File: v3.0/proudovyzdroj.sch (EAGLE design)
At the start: 27 parts, among them IC1 LM358N, Q1 IRF512

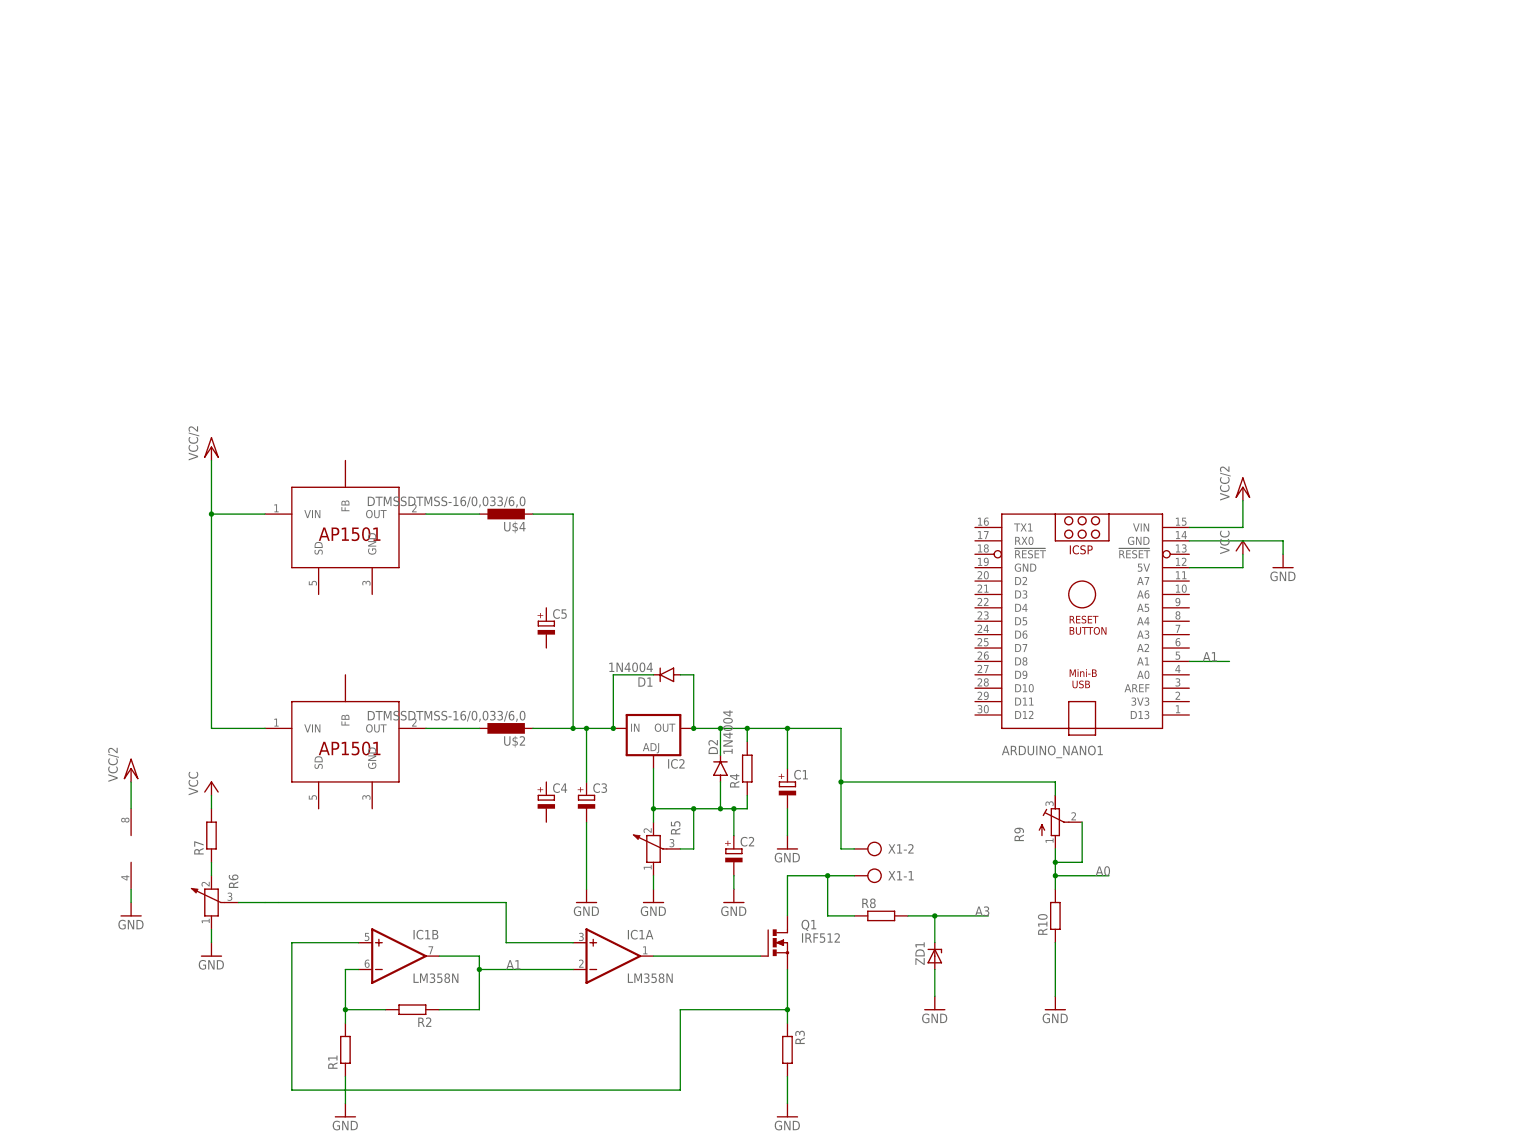
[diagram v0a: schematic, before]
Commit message: základní schéma
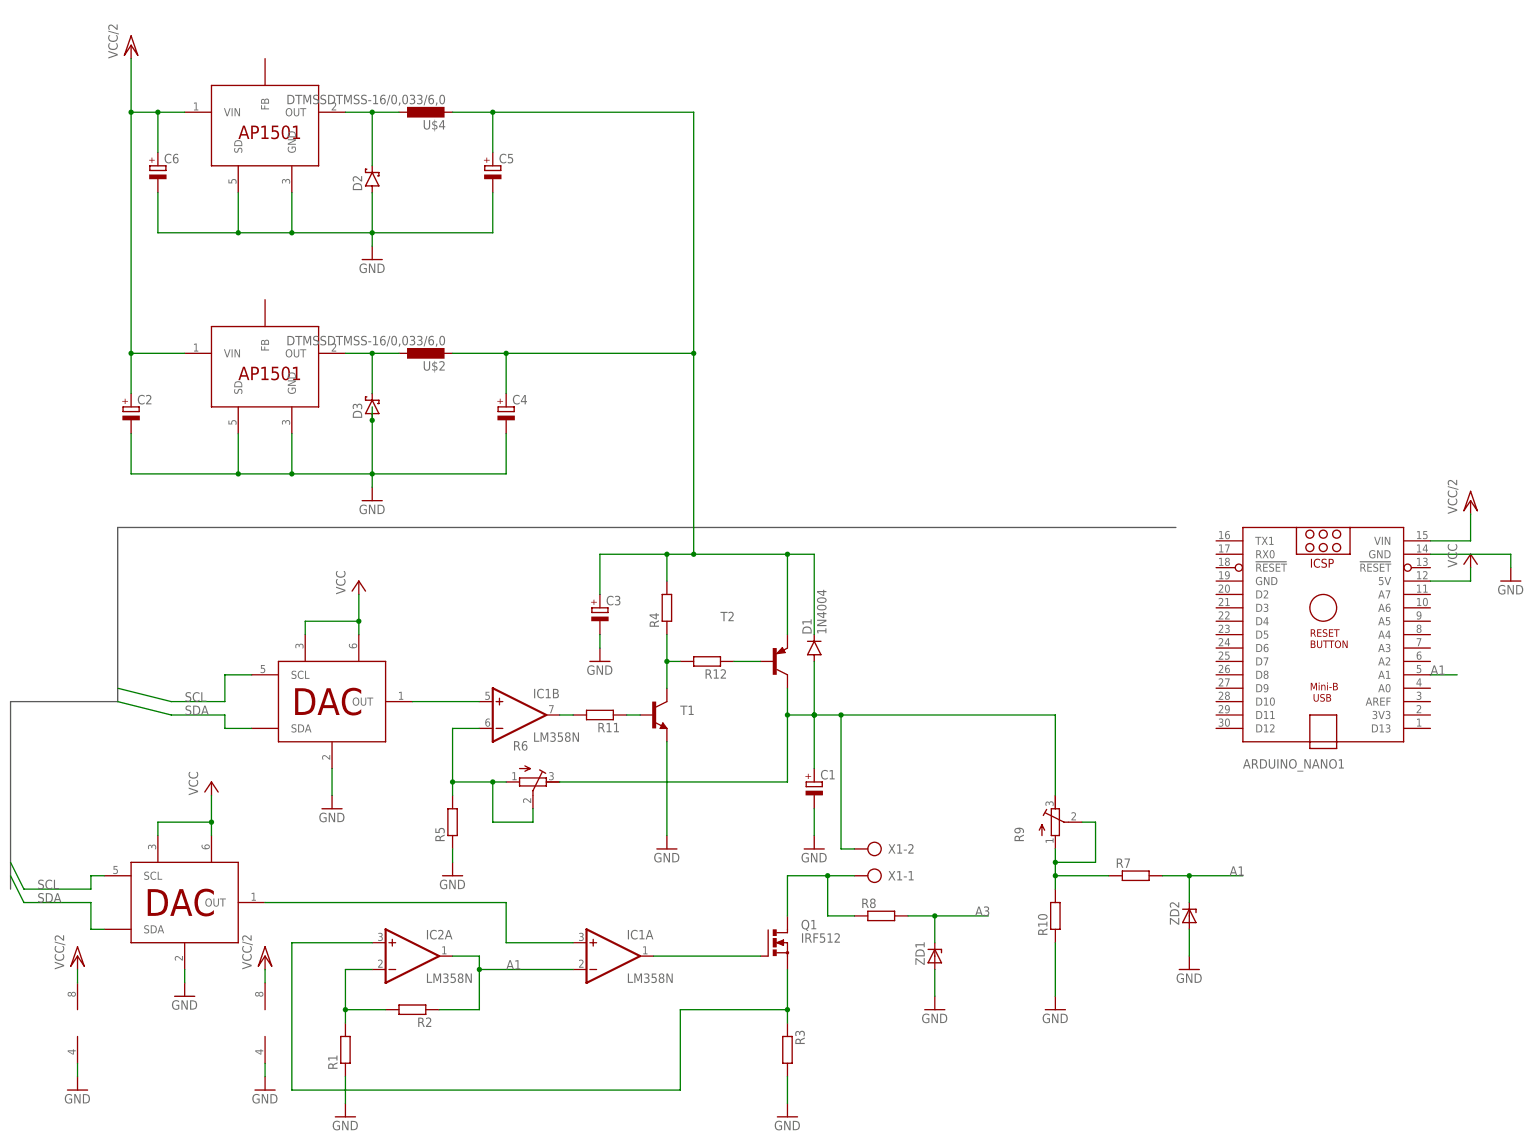
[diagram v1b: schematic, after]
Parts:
- added C6: (no value), rcl:CPOL-EUE3.5-8
- added D3: (no value), diode:SCHOTTKY-DIODESMC
- added R11, R12: (no value), rcl:R-EU_R0805
- added T1: (no value), transistor:BC337-40-NPN-TO92-CBE
- added T2: (no value), transistor-neu-to92:-PNP-TO220V
- added U$5, U$6: MCP4726, DAC:MCP4726
- added ZD2: (no value), devices:DIODE_ZENER5
- D2: value 1N4004 -> (none); device diode:1N4004 -> diode:SCHOTTKY-DIODESMC
- IC2: value (none) -> LM358N; device v-reg:LM317TS -> linear:LM358N
- R5: device rcl:POTENTIOMETER_PT-10S -> rcl:R-EU_R0805
- R6: device rcl:POTENTIOMETER_PT-10S -> rcl:R-TRIMM3339P
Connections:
- removed net A0: R10.2, R9.A, R9.S
- new net N$13: C1.+, D1.A, R6.E, R9.E, T2.C, X1-2.KL
- new net N$14: R12.1, T2.B
- new net N$15: C3.+, C4.+, C5.+, D1.C, R4.2, T2.E, U$2.2, U$4.2
- new net N$16: R12.2, R4.1, T1.C
- new net N$4: R11.1, T1.B
- new net SCL: U$5.SCL, U$6.SCL
- new net SDA: U$5.SDA, U$6.SDA
- net A1: now also IC2A.OUT, R7.2, ZD2.C; no longer IC1B.OUT
- net GND: now also C4.-, C5.-, C6.-, D2.A, D3.A, IC2P.V-, T1.E, U$1.GND, U$1.SD, U$3.GND, U$3.SD, U$5.VSS, U$6.VSS, ZD2.A; no longer R6.1
- net N$1: now also IC2A.+IN; no longer IC1B.+IN
- net N$10: now also D3.C
- net N$11: now also IC1B.-IN, R6.A, R6.S; no longer C2.+, D2.A, IC2.ADJ, R4.1, R5.3
- net N$12: now also IC1B.OUT, R11.2; no longer R6.2, R7.1
- net N$3: now also IC2A.-IN; no longer IC1B.-IN
- net N$5: now also R10.2, R7.1, R9.A, R9.S; no longer C1.+, D1.A, D2.C, IC2.OUT, R4.2, R9.E, X1-2.KL
- net N$6: now also U$5.OUT; no longer R6.3
- net N$8: now also D2.C
- net N$9: now also IC1B.+IN, U$6.OUT; no longer C3.+, D1.C, IC2.IN, U$2.2, U$4.2
- net VCC: now also U$5.VDD, U$5.VREF, U$6.VDD, U$6.VREF; no longer R7.2
- net VCC/2: now also C2.+, C6.+, IC2P.V+
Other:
- moved on the sheet: ARDUINO_NANO1, C1, C2, C3, C4, C5, D1, IC1B, R4, R7, U$2, U$4
